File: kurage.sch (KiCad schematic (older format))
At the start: 106 parts, among them SW1 ESC, SW10 R, SW11 Y, SW12 I, SW13 P, SW14 ], SW15 UNDEFINED2, SW16 CTRL, SW17 A, SW18 D, SW19 G, SW2 Q, SW20 J, SW21 L, SW22 ', SW23 S, SW24 F, SW25 H, SW26 K, SW27 ;, SW28 ENTER, SW29 UNDEFINED3, SW3 E, SW30 LSHIFT, SW31 Z, SW32 C, SW33 B, SW34 M, SW35 ., SW36 RSHIFT, SW37 X, SW38 V, SW39 N, SW4 T, SW40 ,, SW41 /, SW42 UP, SW43 LOWER, SW44 UNDEFINED1, SW45 WIN, SW46 RAISE, SW47 LEFT, SW48 RIGHT, SW49 LSPACE, SW5 U, SW50 RSPACE, SW51 ALT, SW52 DOWN, SW6 O, SW7 [, SW8 BACKSPACE, SW9 W, U1 ProMicro

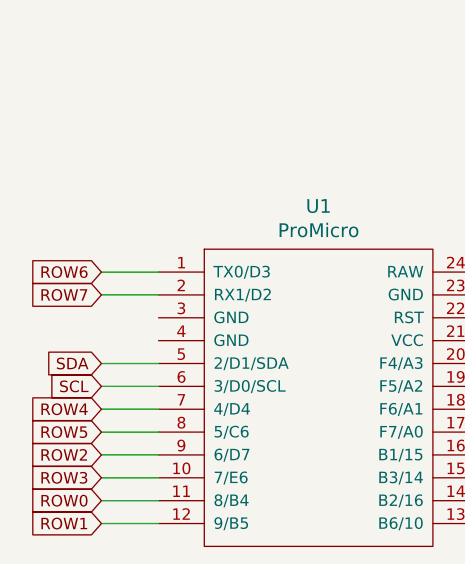
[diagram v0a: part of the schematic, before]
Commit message: progress
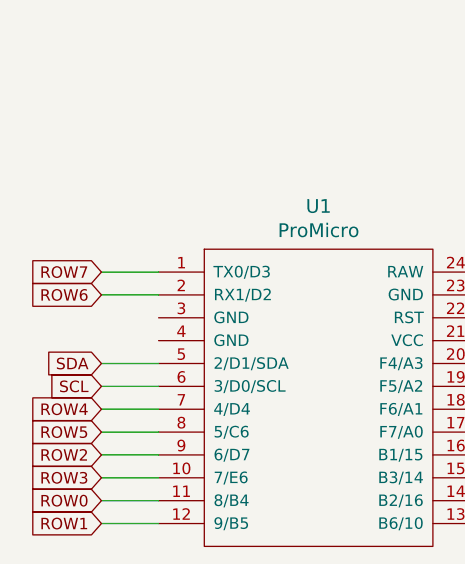
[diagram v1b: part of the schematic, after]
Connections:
- net ROW6: now also U1.2 (RX1/D2); no longer U1.1 (TX0/D3)
- net ROW7: now also U1.1 (TX0/D3); no longer U1.2 (RX1/D2)
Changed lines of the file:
@@
 Text GLabel 1400 6300 0    50   Input ~ 0
 ROW4
+Text GLabel 1400 5700 0    50   Input ~ 0
+ROW7
 Text GLabel 1400 5800 0    50   Input ~ 0
-ROW7
-Text GLabel 1400 5700 0    50   Input ~ 0
 ROW6
 Text GLabel 1400 6700 0    50   Input ~ 0
